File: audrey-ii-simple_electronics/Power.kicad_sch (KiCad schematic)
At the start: 9 parts, among them J1 Conn_02x05_Odd_Even, U5 LM4040DCK-2.0, U6 LD1117S50TR_SOT223

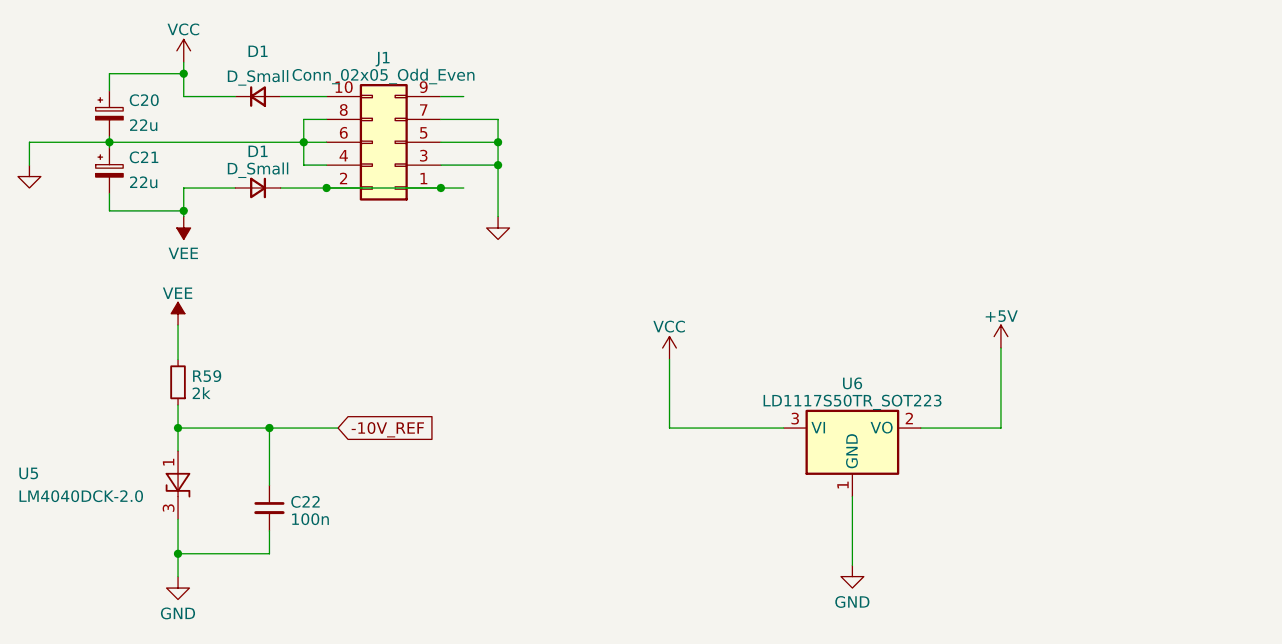
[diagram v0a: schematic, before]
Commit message: -
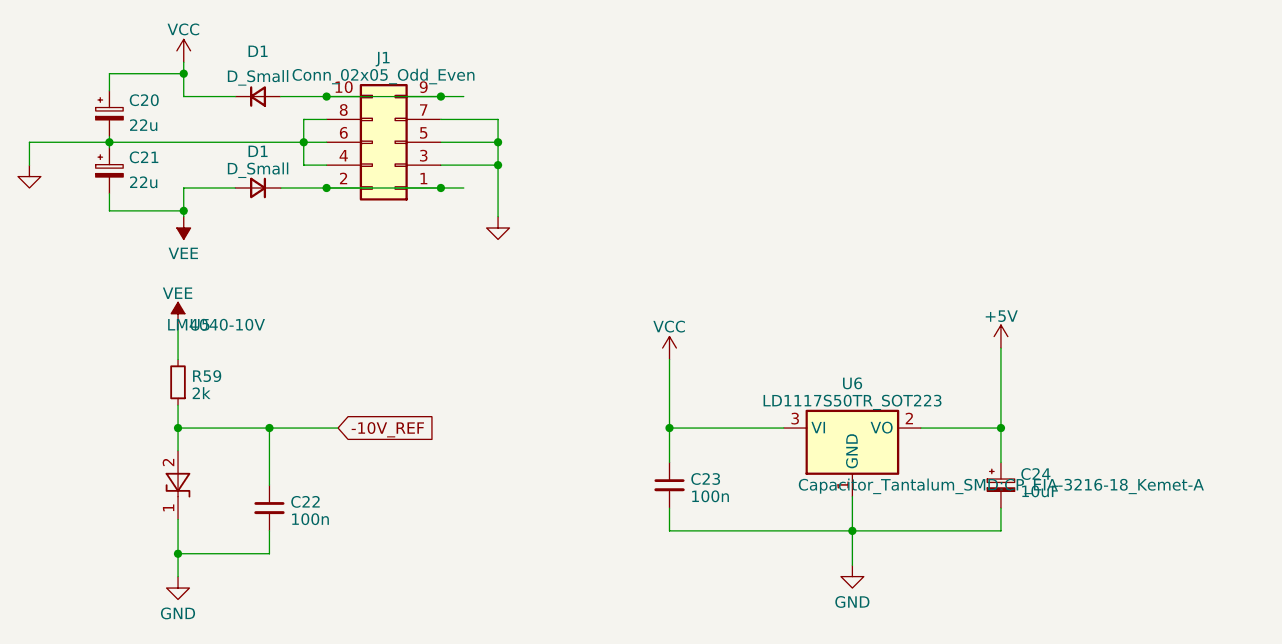
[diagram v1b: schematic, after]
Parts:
- added C23: 100n, Capacitor_SMD:C_0603_1608Metric, symbol Device:C_Small
- added C24: 10uF, Capacitor_Tantalum_SMD:CP_EIA-3216-18_Kemet-A, symbol Device:C_Polarized_Small
- C22: LCSC# (none) -> C14663
- D1: footprint Diode_SMD:D_SOD-123 -> Diode_SMD:D_SMA
- R59: LCSC# (none) -> C22975
- U5: value LM4040DCK-2.0 -> LM4040-10V; footprint Package_TO_SOT_SMD:SOT-353_SC-70-5 -> Package_TO_SOT_SMD:SOT-23-3; LCSC# (none) -> C701887
- U6: LCSC# (none) -> C134077
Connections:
- net +5V: now also C24.1
- net -10V_REF: now also U5.2 (A); no longer U5.1 (A)
- net GND: now also U5.1 (K), C23.2, C24.2; no longer U5.3 (K)
- net VCC: now also C23.1
- net at D1.2 (A), J1.10 (Pin_10): now also J1.9 (Pin_9)
